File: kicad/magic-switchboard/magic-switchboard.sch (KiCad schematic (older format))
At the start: 22 parts, among them Q1 BC547, Q2 BS250, Q3 2N7000, Q4 2N7000, Q5 2N7000, Q6 2N7000, U1 XY-016, U2 alternative Boost Converter

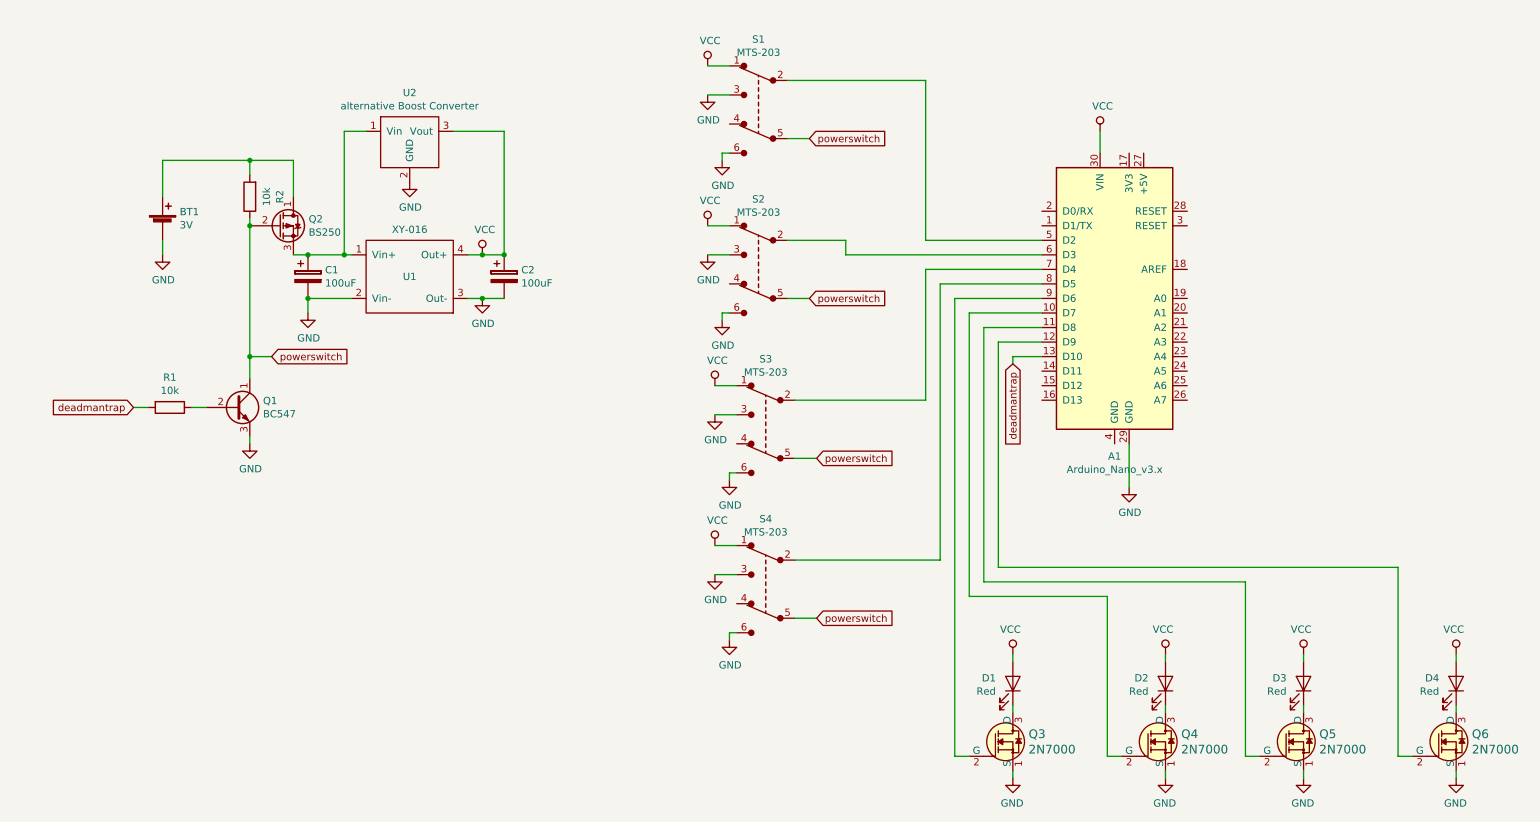
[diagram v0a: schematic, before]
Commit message: attiny2313 board
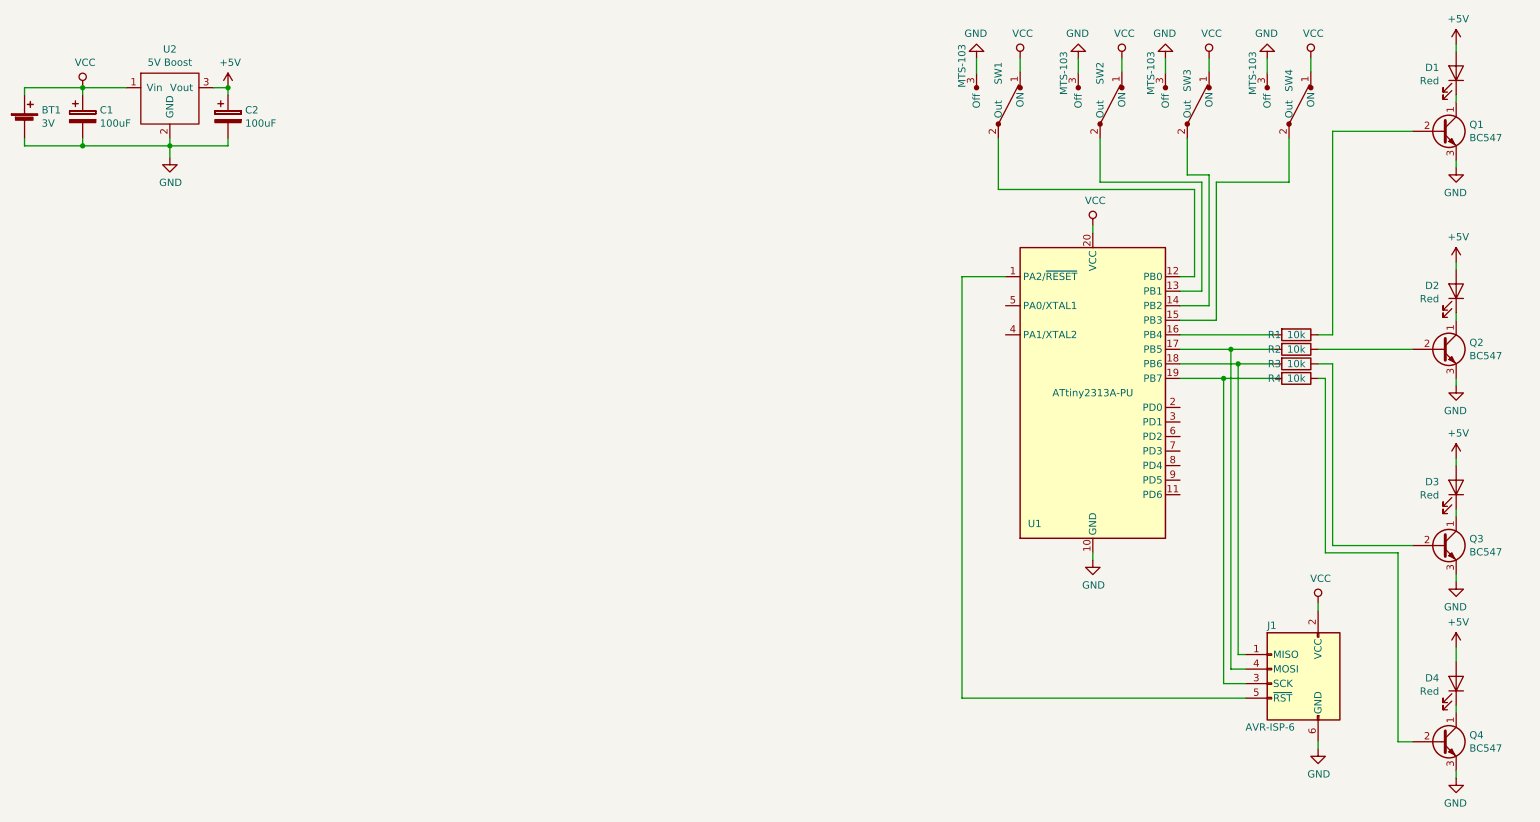
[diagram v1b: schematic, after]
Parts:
- removed A1: Arduino_Nano_v3.x, switchboard:Arduino_Nano, symbol MCU_Module:Arduino_Nano_v3.x
- removed Q2: BS250, switchboard:BS250, symbol Transistor_FET:BS250
- removed Q3, Q4, Q5, Q6: 2N7000, switchboard:2N700, symbol dk_Transistors-FETs-MOSFETs-Single:2N7000
- removed S1, S2, S3, S4: MTS-203, switchboard:MTS-203 Switch, symbol dk_Slide-Switches:JS202011SCQN
- removed U1: XY-016, switchboard:XY-016, symbol switchboard:XY-016
- added J1: AVR-ISP-6, switchboard:ISP6, symbol Connector:AVR-ISP-6
- added Q2, Q3, Q4: BC547, Package_TO_SOT_THT:TO-92_Inline, symbol Transistor_BJT:BC547
- added R3, R4: 10k, switchboard:Resistor, symbol Device:R
- added SW1, SW2, SW3, SW4: MTS-103, switchboard:MTS-103 Switch, symbol switchboard:MTS-103
- added U1: ATtiny2313A-PU, switchboard:ATtiny2313, symbol switchboard:ATtiny2313A-PU
- Q1: footprint switchboard:BC547 -> Package_TO_SOT_THT:TO-92_Inline
- U2: value alternative Boost Converter -> 5V Boost
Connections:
- net GND: now also J1.6 (GND), Q2.3 (E), Q3.3 (E), Q4.3 (E), SW1.3 (Off), SW2.3 (Off), SW3.3 (Off), SW4.3 (Off), U1.10 (GND)
- net VCC: now also BT1.1 (+), C1.1, U2.1 (Vin), J1.2 (VCC), SW1.1 (ON), SW2.1 (ON), SW3.1 (ON), SW4.1 (ON), U1.20 (VCC); no longer C2.1, D1.2 (A), D2.2 (A), D3.2 (A), D4.2 (A), U2.3 (Vout)
- net at R2.2: now also J1.4 (MOSI), U1.17 (PB5); no longer BT1.1 (+)
- net at D2.1 (K): now also Q2.1 (C)
- net at D1.1 (K): now also Q1.1 (C)
- net at D4.1 (K): now also Q4.1 (C)
- net at D3.1 (K): now also Q3.1 (C)
- net deadmantrap: no longer names the net of R1.2
- net deadmantrap: now also U1.16 (PB4)
- net powerswitch: no longer names the net of R2.1
- net powerswitch: now also Q2.2 (B); no longer Q1.1 (C)
- new net: SW1.2 (Out), U1.12 (PB0)
- new net: J1.5 (~RST), U1.1 (PA2/~RESET)
- new net: SW2.2 (Out), U1.13 (PB1)
- new net: SW3.2 (Out), U1.14 (PB2)
- new net: SW4.2 (Out), U1.15 (PB3)
- new net: J1.1 (MISO), R3.2, U1.18 (PB6)
- new net: J1.3 (SCK), R4.2, U1.19 (PB7)
- new net: Q3.2 (B), R3.1
- new net: Q4.2 (B), R4.1
- new net +5V: C2.1, D1.2 (A), D2.2 (A), D3.2 (A), D4.2 (A), U2.3 (Vout)
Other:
- moved on the sheet: BT1, C1, C2, D1, D2, D3, U2
